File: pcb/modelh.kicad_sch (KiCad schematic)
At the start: 46 parts, among them SW1 SW_Push, U1 GD32F103C8T6, U2 AMS1117-3.3, Y1 8MHz

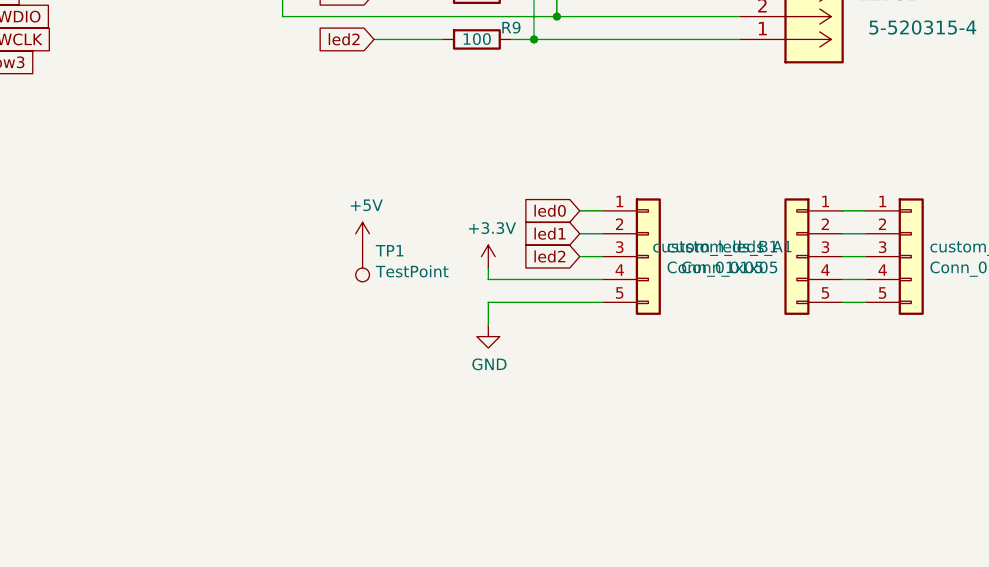
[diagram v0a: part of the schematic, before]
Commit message: Update schematics and pcb
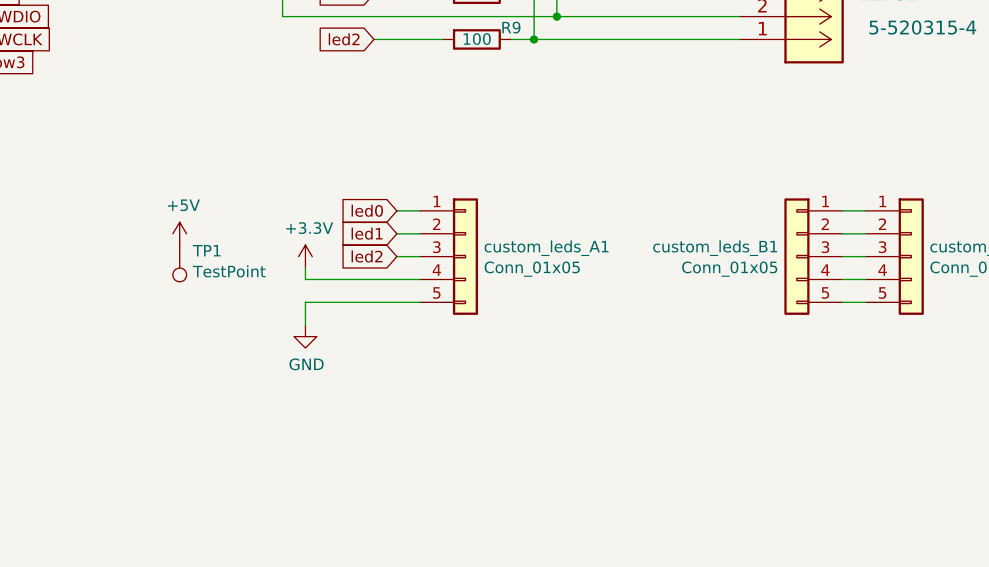
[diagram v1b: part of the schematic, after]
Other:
- moved on the sheet: TP1, custom_leds_A1
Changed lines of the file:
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@@
   (no_connect (at 129.54 83.82))
   (no_connect (at 129.54 81.28))
-  (wire (pts (xy 227.33 151.13) (xy 240.03 151.13))
+  (wire (pts (xy 207.01 151.13) (xy 219.71 151.13))
     (stroke (width 0) (type default) (color 0 0 0 0))
   )
@@
     (stroke (width 0) (type default) (color 0 0 0 0))
   )
-  (wire (pts (xy 227.33 153.67) (xy 240.03 153.67))
+  (wire (pts (xy 207.01 153.67) (xy 219.71 153.67))
     (stroke (width 0) (type default) (color 0 0 0 0))
   )
@@
     (stroke (width 0) (type default) (color 0 0 0 0))
   )
-  (wire (pts (xy 240.03 146.05) (xy 237.49 146.05))
+  (wire (pts (xy 219.71 146.05) (xy 217.17 146.05))
     (stroke (width 0) (type default) (color 0 0 0 0))
   )
@@
     (stroke (width 0) (type default) (color 0 0 0 0))
   )
-  (wire (pts (xy 227.33 151.13) (xy 227.33 149.86))
+  (wire (pts (xy 207.01 151.13) (xy 207.01 149.86))
     (stroke (width 0) (type default) (color 0 0 0 0))
   )
@@
     (stroke (width 0) (type default) (color 0 0 0 0))
   )
-  (wire (pts (xy 240.03 143.51) (xy 237.49 143.51))
+  (wire (pts (xy 219.71 143.51) (xy 217.17 143.51))
     (stroke (width 0) (type default) (color 0 0 0 0))
   )
@@
     (stroke (width 0) (type default) (color 0 0 0 0))
   )
-  (wire (pts (xy 237.49 148.59) (xy 240.03 148.59))
+  (wire (pts (xy 217.17 148.59) (xy 219.71 148.59))
     (stroke (width 0) (type default) (color 0 0 0 0))
   )
@@
     (stroke (width 0) (type default) (color 0 0 0 0))
   )
-  (wire (pts (xy 227.33 153.67) (xy 227.33 156.21))
+  (wire (pts (xy 207.01 153.67) (xy 207.01 156.21))
     (stroke (width 0) (type default) (color 0 0 0 0))
   )
@@
     )
   )
-  (global_label "led2" (shape input) (at 237.49 148.59 180) (fields_autoplaced)
-    (effects (font (size 1.27 1.27)) (justify right))
-    (property "Intersheet References" "${INTERSHEET_REFS}" (id 0) (at 0 0 0)
+  (global_label "led2" (shape input) (at 217.17 148.59 180) (fields_autoplaced)
+    (effects (font (size 1.27 1.27)) (justify right))
+    (property "Intersheet References" "${INTERSHEET_REFS}" (id 0) (at -20.32 0 0)
       (effects (font (size 1.27 1.27)) hide)
     )
@@
     )
   )
-  (global_label "led1" (shape input) (at 237.49 146.05 180) (fields_autoplaced)
-    (effects (font (size 1.27 1.27)) (justify right))
-    (property "Intersheet References" "${INTERSHEET_REFS}" (id 0) (at 0 0 0)
+  (global_label "led1" (shape input) (at 217.17 146.05 180) (fields_autoplaced)
+    (effects (font (size 1.27 1.27)) (justify right))
+    (property "Intersheet References" "${INTERSHEET_REFS}" (id 0) (at -20.32 0 0)
       (effects (font (size 1.27 1.27)) hide)
     )
@@
     )
   )
-  (global_label "led0" (shape input) (at 237.49 143.51 180) (fields_autoplaced)
-    (effects (font (size 1.27 1.27)) (justify right))
-    (property "Intersheet References" "${INTERSHEET_REFS}" (id 0) (at 0 0 0)
+  (global_label "led0" (shape input) (at 217.17 143.51 180) (fields_autoplaced)
+    (effects (font (size 1.27 1.27)) (justify right))
+    (property "Intersheet References" "${INTERSHEET_REFS}" (id 0) (at -20.32 0 0)
       (effects (font (size 1.27 1.27)) hide)
     )
@@
     (pin "2")
   )
-  (symbol (lib_id "power:+3.3V") (at 227.33 149.86 0) (unit 1)
-    (in_bom yes) (on_board yes)
-    (property "Reference" "#PWR0119" (id 0) (at 227.33 153.67 0)
-      (effects (font (size 1.27 1.27)) hide)
-    )
-    (property "Value" "+3.3V" (id 1) (at 227.711 145.4658 0))
-    (property "Footprint" "" (id 2) (at 227.33 149.86 0)
-      (effects (font (size 1.27 1.27)) hide)
-    )
-    (property "Datasheet" "" (id 3) (at 227.33 149.86 0)
+  (symbol (lib_id "power:+3.3V") (at 207.01 149.86 0) (unit 1)
+    (in_bom yes) (on_board yes)
+    (property "Reference" "#PWR0119" (id 0) (at 207.01 153.67 0)
+      (effects (font (size 1.27 1.27)) hide)
+    )
+    (property "Value" "+3.3V" (id 1) (at 207.391 145.4658 0))
+    (property "Footprint" "" (id 2) (at 207.01 149.86 0)
+      (effects (font (size 1.27 1.27)) hide)
+    )
+    (property "Datasheet" "" (id 3) (at 207.01 149.86 0)
       (effects (font (size 1.27 1.27)) hide)
     )
@@
     (pin "2")
   )
-  (symbol (lib_id "power:GND") (at 227.33 156.21 0) (unit 1)
-    (in_bom yes) (on_board yes)
-    (property "Reference" "#PWR0125" (id 0) (at 227.33 162.56 0)
-      (effects (font (size 1.27 1.27)) hide)
-    )
-    (property "Value" "GND" (id 1) (at 227.457 160.6042 0))
-    (property "Footprint" "" (id 2) (at 227.33 156.21 0)
-      (effects (font (size 1.27 1.27)) hide)
-    )
-    (property "Datasheet" "" (id 3) (at 227.33 156.21 0)
+  (symbol (lib_id "power:GND") (at 207.01 156.21 0) (unit 1)
+    (in_bom yes) (on_board yes)
+    (property "Reference" "#PWR0125" (id 0) (at 207.01 162.56 0)
+      (effects (font (size 1.27 1.27)) hide)
+    )
+    (property "Value" "GND" (id 1) (at 207.137 160.6042 0))
+    (property "Footprint" "" (id 2) (at 207.01 156.21 0)
+      (effects (font (size 1.27 1.27)) hide)
+    )
+    (property "Datasheet" "" (id 3) (at 207.01 156.21 0)
       (effects (font (size 1.27 1.27)) hide)
     )
@@
     (pin "5")
   )
-  (symbol (lib_id "Connector:TestPoint") (at 213.36 147.32 180) (unit 1)
-    (in_bom yes) (on_board yes)
-    (property "Reference" "TP1" (id 0) (at 214.8332 147.9804 0)
+  (symbol (lib_id "Connector:TestPoint") (at 193.04 147.32 180) (unit 1)
+    (in_bom yes) (on_board yes)
+    (property "Reference" "TP1" (id 0) (at 194.5132 147.9804 0)
       (effects (font (size 1.27 1.27)) (justify right))
     )
-    (property "Value" "TestPoint" (id 1) (at 214.8332 150.2918 0)
+    (property "Value" "TestPoint" (id 1) (at 194.5132 150.2918 0)
       (effects (font (size 1.27 1.27)) (justify right))
     )
-    (property "Footprint" "TestPoint:TestPoint_THTPad_D1.5mm_Drill0.7mm" (id 2) (at 208.28 147.32 0)
-      (effects (font (size 1.27 1.27)) hide)
-    )
-    (property "Datasheet" "~" (id 3) (at 208.28 147.32 0)
+    (property "Footprint" "TestPoint:TestPoint_THTPad_D1.5mm_Drill0.7mm" (id 2) (at 187.96 147.32 0)
+      (effects (font (size 1.27 1.27)) hide)
+    )
+    (property "Datasheet" "~" (id 3) (at 187.96 147.32 0)
       (effects (font (size 1.27 1.27)) hide)
     )
@@
     (pin "3")
   )
-  (symbol (lib_id "power:+5V") (at 213.36 147.32 0) (unit 1)
-    (in_bom yes) (on_board yes)
-    (property "Reference" "#PWR0126" (id 0) (at 213.36 151.13 0)
-      (effects (font (size 1.27 1.27)) hide)
-    )
-    (property "Value" "+5V" (id 1) (at 213.741 142.9258 0))
-    (property "Footprint" "" (id 2) (at 213.36 147.32 0)
-      (effects (font (size 1.27 1.27)) hide)
-    )
-    (property "Datasheet" "" (id 3) (at 213.36 147.32 0)
+  (symbol (lib_id "power:+5V") (at 193.04 147.32 0) (unit 1)
+    (in_bom yes) (on_board yes)
+    (property "Reference" "#PWR0126" (id 0) (at 193.04 151.13 0)
+      (effects (font (size 1.27 1.27)) hide)
+    )
+    (property "Value" "+5V" (id 1) (at 193.421 142.9258 0))
+    (property "Footprint" "" (id 2) (at 193.04 147.32 0)
+      (effects (font (size 1.27 1.27)) hide)
+    )
+    (property "Datasheet" "" (id 3) (at 193.04 147.32 0)
       (effects (font (size 1.27 1.27)) hide)
     )
@@
     (pin "2")
   )
-  (symbol (lib_id "Connector_Generic:Conn_01x05") (at 245.11 148.59 0) (unit 1)
-    (in_bom yes) (on_board yes)
-    (property "Reference" "custom_leds_A1" (id 0) (at 247.142 147.5232 0)
-      (effects (font (size 1.27 1.27)) (justify left))
-    )
-    (property "Value" "Conn_01x05" (id 1) (at 247.142 149.8346 0)
-      (effects (font (size 1.27 1.27)) (justify left))
-    )
-    (property "Footprint" "Connector_PinSocket_2.54mm:PinSocket_1x05_P2.54mm_Vertical" (id 2) (at 245.11 148.59 0)
-      (effects (font (size 1.27 1.27)) hide)
-    )
-    (property "Datasheet" "~" (id 3) (at 245.11 148.59 0)
-      (effects (font (size 1.27 1.27)) hide)
-    )
+  (symbol (lib_id "Connector_Generic:Conn_01x05") (at 224.79 148.59 0) (unit 1)
+    (in_bom yes) (on_board yes)
+    (property "Reference" "custom_leds_A1" (id 0) (at 226.822 147.5232 0)
+      (effects (font (size 1.27 1.27)) (justify left))
+    )
+    (property "Value" "Conn_01x05" (id 1) (at 226.822 149.8346 0)
+      (effects (font (size 1.27 1.27)) (justify left))
+    )
+    (property "Footprint" "Connector_PinSocket_2.54mm:PinSocket_1x05_P2.54mm_Vertical" (id 2) (at 224.79 148.59 0)
+      (effects (font (size 1.27 1.27)) hide)
+    )
+    (property "Datasheet" "~" (id 3) (at 224.79 148.59 0)
+      (effects (font (size 1.27 1.27)) hide)
+    )
